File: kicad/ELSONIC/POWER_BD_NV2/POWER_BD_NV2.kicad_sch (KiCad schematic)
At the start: 40 parts, among them J1 SMW250-02P, J2 SMW250-06P, J3 TAP_250, J5 TAP_250, U1 ICE3BR0665J, U2 PC817

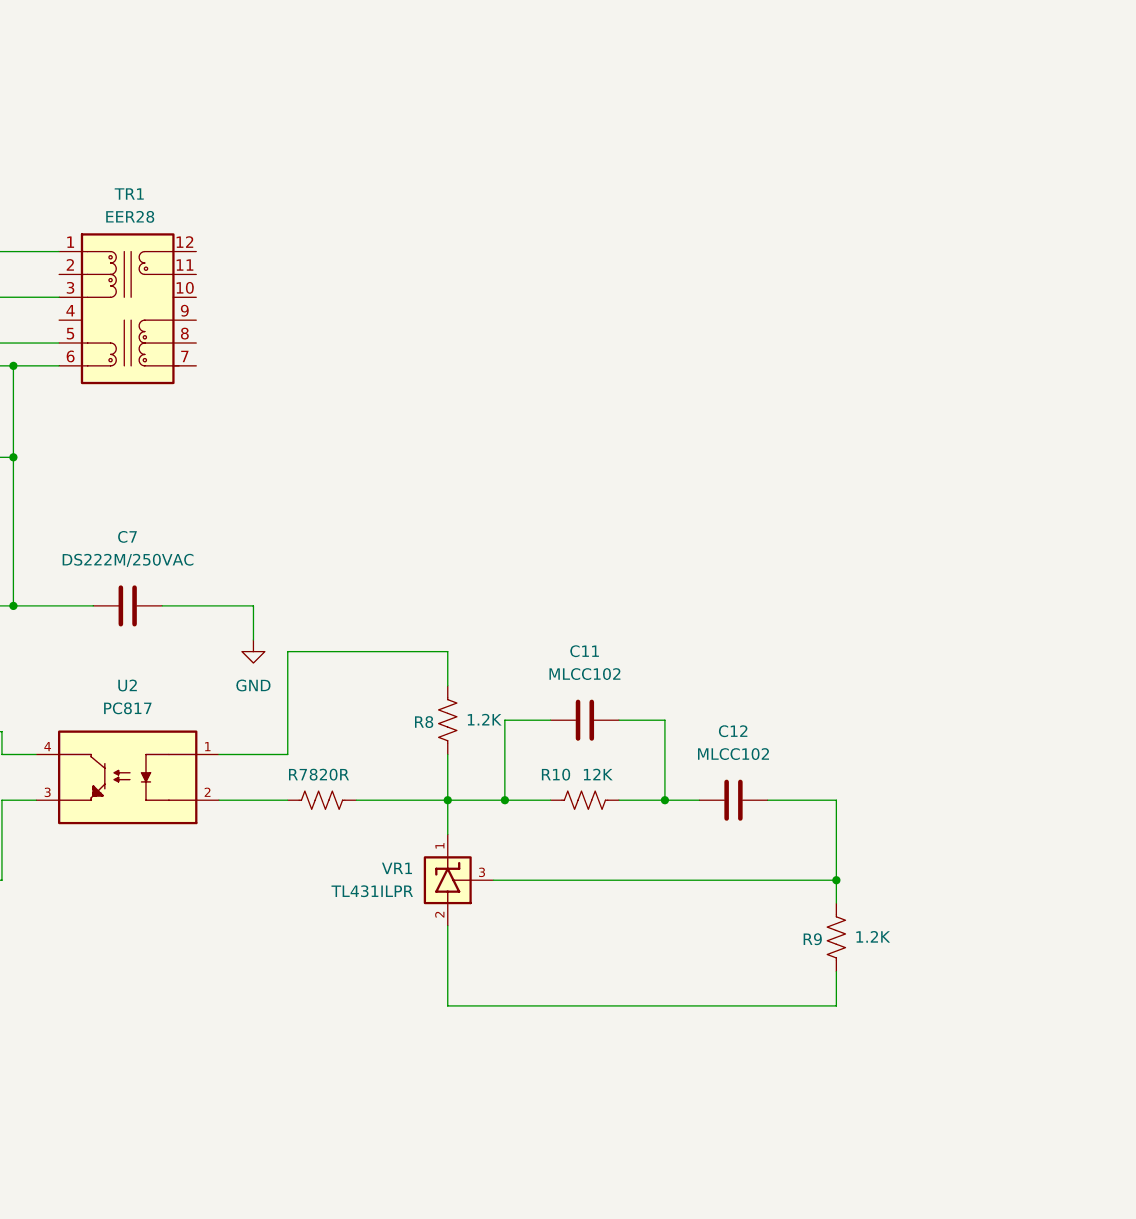
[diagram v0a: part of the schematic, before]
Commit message: Update KiCAD schematic and library files
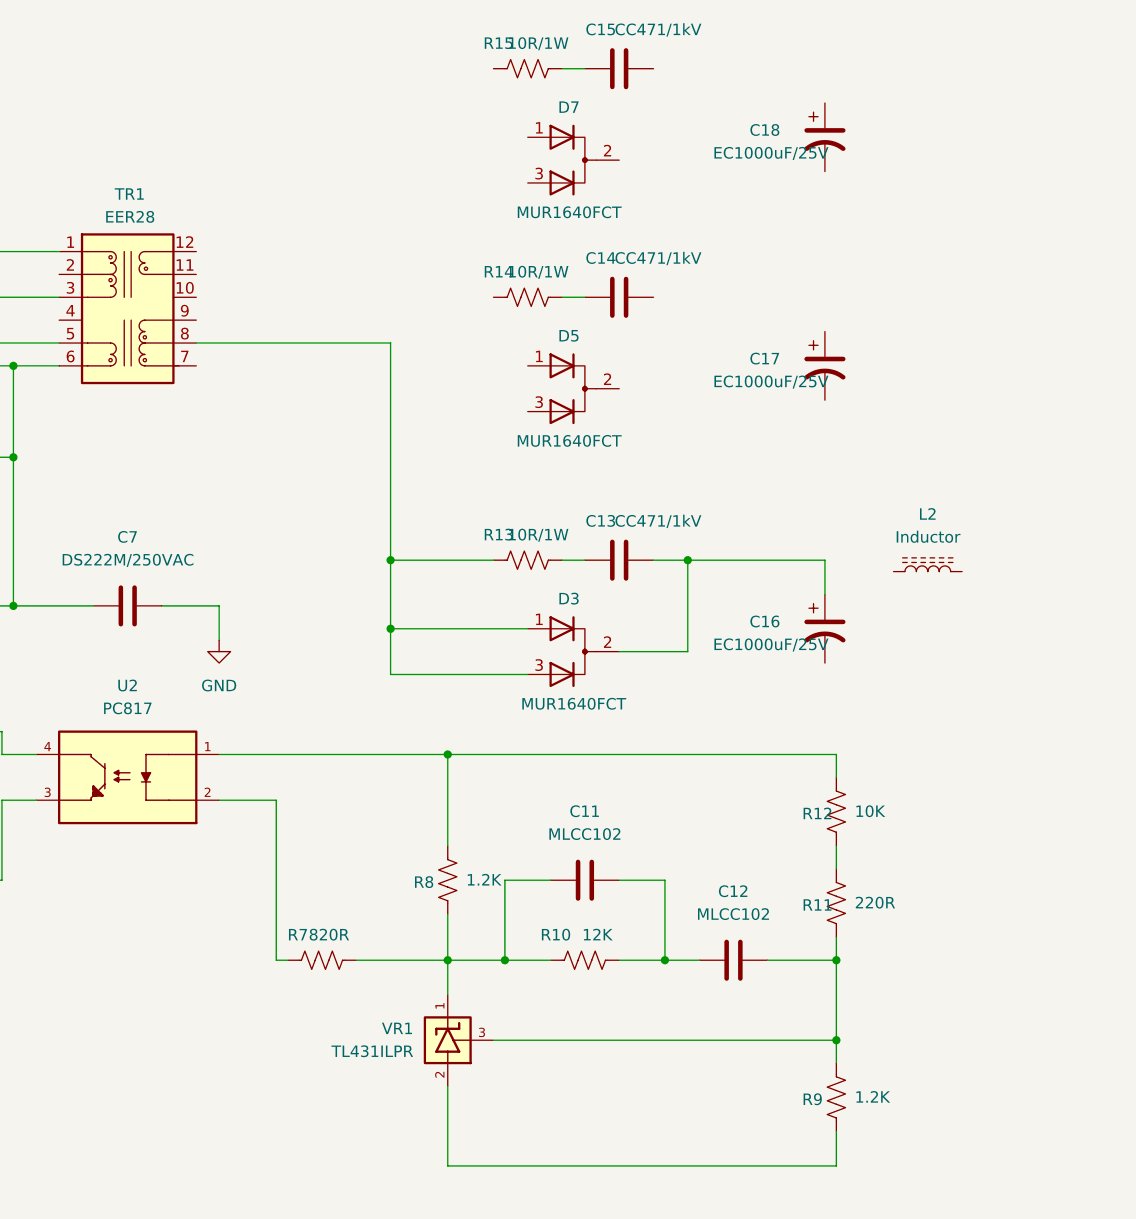
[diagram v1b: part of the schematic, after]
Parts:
- added C13, C14, C15: CC471/1kV, symbol 04_MyLib_Passive:C
- added C16, C17, C18: EC1000uF/25V, symbol 04_MyLib_Passive:C_Pol
- added D3, D5, D7: MUR1640FCT, 03_MyFoot_Active:TO255P510X1070X2140-3P, symbol 03_MyLib_Active:MUR1640FCT
- added L2: Inductor, symbol 04_MyLib_Passive:Inductor
- added R11: 220R, 04_MyFoot_Passive:R_Axial_P10.16mm, symbol 04_MyLib_Passive:R
- added R12: 10K, 04_MyFoot_Passive:R_Axial_P10.16mm, symbol 04_MyLib_Passive:R
- added R13, R14, R15: 10R/1W, 04_MyFoot_Passive:R_Axial_P10.16mm, symbol 04_MyLib_Passive:R
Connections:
- net at C12.2, R9.2, VR1.3: now also R11.1
- net at TR1.8 (N1): now also D3.1 (A), D3.3 (A), R13.1
- net at R8.2, U2.1: now also R12.2
- new net: C13.2, C16.1, D3.2 (K)
- new net: R11.2, R12.1
- new net: C13.1, R13.2
- new net: C15.1, R15.2
- new net: C14.1, R14.2
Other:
- moved on the sheet: C11, C12, R10, R7, R8, R9, VR1
